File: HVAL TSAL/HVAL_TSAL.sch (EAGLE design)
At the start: 17 parts, among them IC1-LM555 LM555N, X1 22-23-2021

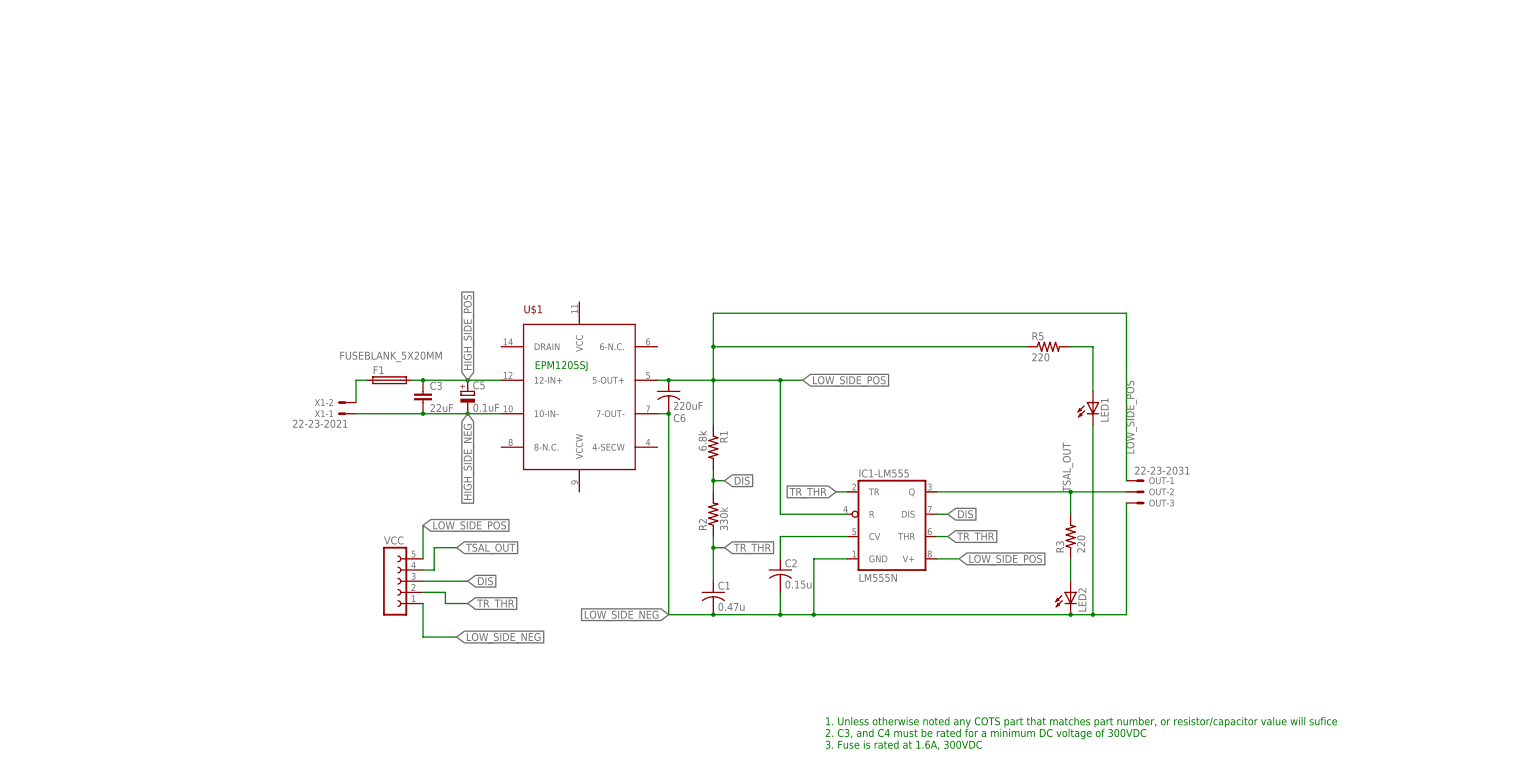
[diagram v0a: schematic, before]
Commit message: Brandon update.
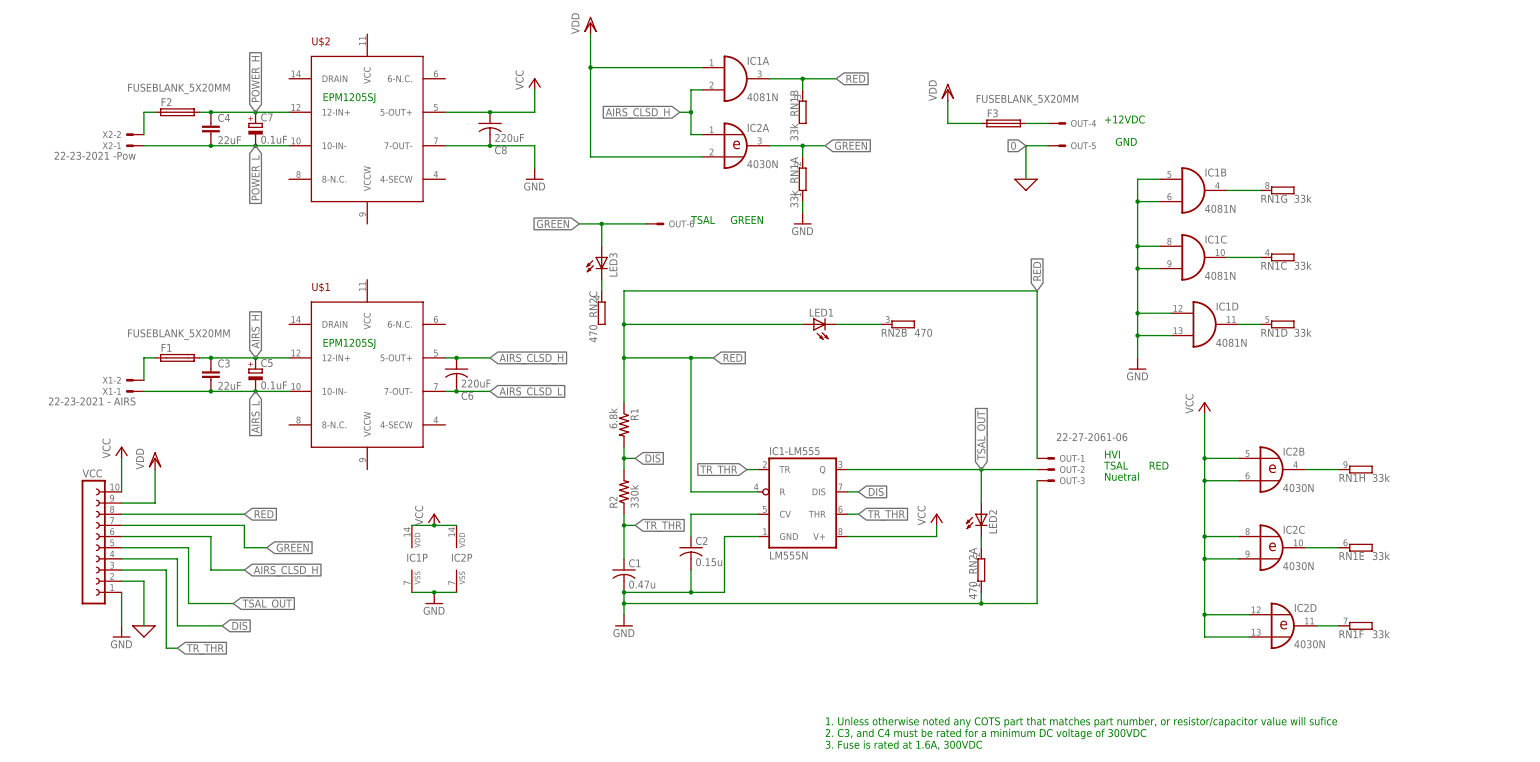
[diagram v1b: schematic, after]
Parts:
- removed R3, R5: 220, resistor:R-US_0309/12
- added C4: 22uF, rcl:C-EU150-091X182
- added C7: 0.1uF, rcl:CPOL-EUE7.5-16
- added C8: 220uF, rcl:C-US050-055X075
- added F2, F3: FUSEBLANK_5X20MM, fuse:FUSEBLANK_5X20MM
- added IC1: 4081N, 40xx:4081N
- added IC2: 4030N, 40xx:4030N
- added LED3: (no value), led:LED3MM
- added RN1: 33k, resistor-sil:GE08R
- added RN2: 470, resistor-sil:GE03R
- added U$2: EPM1205SJ, DC-DC Converter:EPM1205SJ
- added X2: 22-23-2021 -Pow, con-molex:22-23-2021
- OUT: value 22-23-2031 -> 22-27-2061-06; device con-molex:22-23-2031 -> con-molex:22-27-2061-06
- VCC: device con-lsta:FE05W -> con-lsta:FE10-1
- X1: value 22-23-2021 -> 22-23-2021 - AIRS
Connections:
- net HIGH_SIDE_NEG renamed AIRS_L
- net HIGH_SIDE_POS renamed AIRS_H
- removed net LOW_SIDE_NEG: C1.2, C2.2, C6.2, IC1-LM555.GND, LED1.C, LED2.C, OUT-3.S, U$1.7-OUT-, VCC.1
- removed net LOW_SIDE_POS: C6.1, IC1-LM555.R, IC1-LM555.V+, OUT-1.S, R1.1, R5.1, U$1.5-OUT+, VCC.5
- removed net TSAL_IN: LED1.A, R5.2
- new net 0: OUT-5.S, VCC.2
- new net AIRS_CLSD_H: C6.1, IC1A.I1, IC2A.I0, U$1.5-OUT+, VCC.6
- new net AIRS_CLSD_L: C6.2, U$1.7-OUT-
- new net GND: C1.2, C2.2, C8.2, IC1-LM555.GND, IC1B.I0, IC1B.I1, IC1C.I0, IC1C.I1, IC1D.I0, IC1D.I1, IC1P.VSS, IC2P.VSS, OUT-3.S, RN1A.1, RN2A.1, U$2.7-OUT-, VCC.1
- new net GREEN: IC2A.O, LED3.A, OUT-6.S, RN1A.2, VCC.7
- new net N$11: IC2D.O, RN1F.2
- new net N$14: LED1.C, RN2B.2
- new net N$15: LED3.C, RN2C.2
- new net N$2: IC2C.O, RN1E.2
- new net N$3: IC1D.O, RN1D.2
- new net N$4: F2.1, X2-2.S
- new net N$5: F3.2, OUT-4.S
- new net N$6: IC1C.O, RN1C.2
- new net N$8: IC2B.O, RN1H.2
- new net N$9: IC1B.O, RN1G.2
- new net POWER_H: C4.1, C7.+, F2.2, U$2.12-IN+
- new net POWER_L: C4.2, C7.-, U$2.10-IN-, X2-1.S
- new net RED: IC1-LM555.R, IC1A.O, LED1.A, OUT-1.S, R1.1, RN1B.2, VCC.8
- new net VCC: C8.1, IC1-LM555.V+, IC1P.VDD, IC2B.I0, IC2B.I1, IC2C.I0, IC2C.I1, IC2D.I0, IC2D.I1, IC2P.VDD, U$2.5-OUT+, VCC.10
- new net VDD: F3.1, IC1A.I0, IC2A.I1, VCC.9
- net DIS: now also VCC.4; no longer VCC.3
- net N$1: now also LED2.C, RN2A.2; no longer LED2.A, R3.1
- net TR_THR: now also VCC.3; no longer VCC.2
- net TSAL_OUT: now also LED2.A, VCC.5; no longer R3.2, VCC.4
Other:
- note added: "+12VDC"
- note added: "GND"
- note added: "HVI"
- note added: "Nuetral"
- note added: "RED"
- note added: "TSAL"
- note added: "TSAL GREEN"
- moved on the sheet: C1, C2, C3, C5, C6, F1, IC1-LM555, LED1, LED2, OUT-1, OUT-2, OUT-3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
